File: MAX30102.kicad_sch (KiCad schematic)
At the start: 7 parts, among them U4 MAX30102, U7 AZ1117-1.8

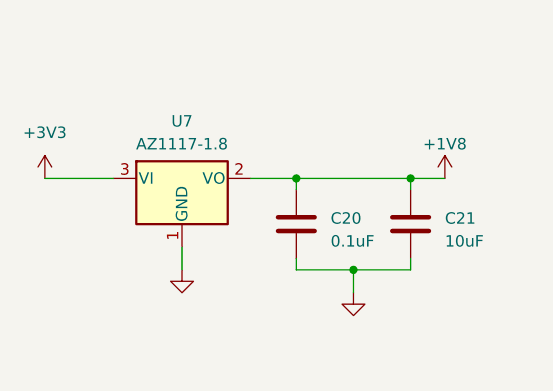
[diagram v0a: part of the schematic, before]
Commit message: Final Design
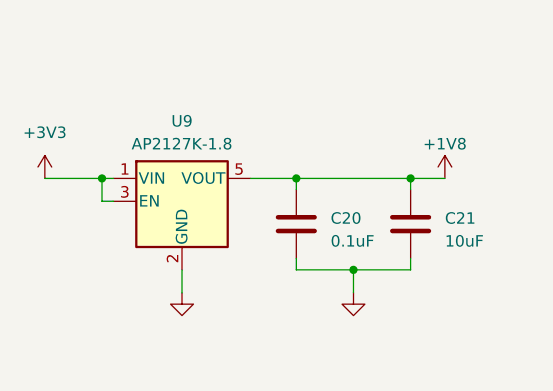
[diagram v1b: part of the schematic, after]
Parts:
- removed U7: AZ1117-1.8, Package_TO_SOT_SMD:SOT-89-3, symbol Regulator_Linear:AZ1117-1.8
- added U9: AP2127K-1.8, Package_TO_SOT_SMD:SOT-23-5, symbol Regulator_Linear:AP2127K-1.8
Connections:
- net +1V8: now also U9.5 (VOUT)
- net +3V3: now also U9.1 (VIN), U9.3 (EN)
- net GND: now also U9.2 (GND)
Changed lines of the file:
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@@
   (junction (at 181.61 106.68) (diameter 0) (color 0 0 0 0)
   )
+  (junction (at 91.44 102.87) (diameter 0) (color 0 0 0 0)
+  )
   (junction (at 181.61 104.14) (diameter 0) (color 0 0 0 0)
   )
   (junction (at 125.73 102.87) (diameter 0) (color 0 0 0 0)
   )
+  (wire (pts (xy 91.44 105.41) (xy 91.44 102.87))
+    (stroke (width 0) (type default))
+  )
   (wire (pts (xy 181.61 113.03) (xy 181.61 106.68))
     (stroke (width 0) (type default))
@@
     (stroke (width 0) (type default))
   )
-  (wire (pts (xy 85.09 102.87) (xy 92.71 102.87))
+  (wire (pts (xy 92.71 105.41) (xy 91.44 105.41))
+    (stroke (width 0) (type default))
+  )
+  (wire (pts (xy 85.09 102.87) (xy 91.44 102.87))
     (stroke (width 0) (type default))
   )
@@
     (stroke (width 0) (type default))
   )
-  (wire (pts (xy 100.33 113.03) (xy 100.33 110.49))
-    (stroke (width 0) (type default))
-  )
   (wire (pts (xy 129.54 102.87) (xy 125.73 102.87))
     (stroke (width 0) (type default))
@@
     (stroke (width 0) (type default))
   )
+  (wire (pts (xy 91.44 102.87) (xy 92.71 102.87))
+    (stroke (width 0) (type default))
+  )
   (wire (pts (xy 113.03 104.14) (xy 113.03 102.87))
     (stroke (width 0) (type default))
@@
   )
   (wire (pts (xy 209.55 106.68) (xy 215.9 106.68))
+    (stroke (width 0) (type default))
+  )
+  (wire (pts (xy 100.33 113.03) (xy 100.33 115.57))
     (stroke (width 0) (type default))
   )
@@
     )
   )
-  (symbol (lib_id "Regulator_Linear:AZ1117-1.8") (at 100.33 102.87 0) (unit 1)
-    (in_bom yes) (on_board yes) (dnp no) (fields_autoplaced)
-    (property "Reference" "U7" (at 100.33 96.52 0)
-      (effects (font (size 1.27 1.27)))
-    )
-    (property "Value" "AZ1117-1.8" (at 100.33 99.06 0)
-      (effects (font (size 1.27 1.27)))
-    )
-    (property "Footprint" "Package_TO_SOT_SMD:SOT-89-3" (at 100.33 96.52 0)
-      (effects (font (size 1.27 1.27) italic) hide)
-    )
-    (property "Datasheet" "https://www.diodes.com/assets/Datasheets/AZ1117.pdf" (at 100.33 102.87 0)
-      (effects (font (size 1.27 1.27)) hide)
-    )
-    (pin "1")
-    (pin "2")
-    (pin "3")
-    (instances
-      (project "RP2040_SOS_band"
-        (path "/1d911b84-17e1-4d47-ac8f-a730104b53ed/d354c91b-03e4-4b78-829b-33cd8f15be96"
-          (reference "U7") (unit 1)
-        )
-      )
-    )
-  )
   (symbol (lib_id "Device:C") (at 113.03 107.95 0) (unit 1)
     (in_bom yes) (on_board yes) (dnp no) (fields_autoplaced)
@@
         (path "/1d911b84-17e1-4d47-ac8f-a730104b53ed/d354c91b-03e4-4b78-829b-33cd8f15be96"
           (reference "#PWR041") (unit 1)
+        )
+      )
+    )
+  )
+  (symbol (lib_id "Regulator_Linear:AP2127K-1.8") (at 100.33 105.41 0) (unit 1)
+    (in_bom yes) (on_board yes) (dnp no) (fields_autoplaced)
+    (property "Reference" "U9" (at 100.33 96.52 0)
+      (effects (font (size 1.27 1.27)))
+    )
+    (property "Value" "AP2127K-1.8" (at 100.33 99.06 0)
+      (effects (font (size 1.27 1.27)))
+    )
+    (property "Footprint" "Package_TO_SOT_SMD:SOT-23-5" (at 100.33 97.155 0)
+      (effects (font (size 1.27 1.27)) hide)
+    )
+    (property "Datasheet" "https://www.diodes.com/assets/Datasheets/AP2127.pdf" (at 100.33 102.87 0)
+      (effects (font (size 1.27 1.27)) hide)
+    )
+    (pin "1")
+    (pin "2")
+    (pin "3")
+    (pin "4")
+    (pin "5")
+    (instances
+      (project "RP2040_SOS_band"
+        (path "/1d911b84-17e1-4d47-ac8f-a730104b53ed/892de33d-264e-4bda-a61c-c8174f81e463"
+          (reference "U9") (unit 1)
+        )
+        (path "/1d911b84-17e1-4d47-ac8f-a730104b53ed/d354c91b-03e4-4b78-829b-33cd8f15be96"
+          (reference "U7") (unit 1)
         )
       )
@@
     )
   )
-  (symbol (lib_id "power:GND") (at 100.33 113.03 0) (unit 1)
-    (in_bom yes) (on_board yes) (dnp no) (fields_autoplaced)
-    (property "Reference" "#PWR031" (at 100.33 119.38 0)
-      (effects (font (size 1.27 1.27)) hide)
-    )
-    (property "Value" "GND" (at 100.33 118.11 0)
-      (effects (font (size 1.27 1.27)) hide)
-    )
-    (property "Footprint" "" (at 100.33 113.03 0)
-      (effects (font (size 1.27 1.27)) hide)
-    )
-    (property "Datasheet" "" (at 100.33 113.03 0)
-      (effects (font (size 1.27 1.27)) hide)
-    )
+  (symbol (lib_id "power:GND") (at 100.33 115.57 0) (unit 1)
+    (in_bom yes) (on_board yes) (dnp no) (fields_autoplaced)
+    (property "Reference" "#PWR031" (at 100.33 121.92 0)
+      (effects (font (size 1.27 1.27)) hide)
+    )
+    (property "Value" "GND" (at 100.33 120.65 0)
+      (effects (font (size 1.27 1.27)) hide)
+    )
+    (property "Footprint" "" (at 100.33 115.57 0)
+      (effects (font (size 1.27 1.27)) hide)
+    )
+    (property "Datasheet" "" (at 100.33 115.57 0)
+      (effects (font (size 1.27 1.27)) hide)
+    )
